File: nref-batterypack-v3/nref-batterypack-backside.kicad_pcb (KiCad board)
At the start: 2 copper layers, 75 x 17 mm, 8 parts, among them J1 C1+, J2 C2-, J3 C3+, J4 C4-, J5 FRONT_CONN

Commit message: battpack v3 snapshot
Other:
- board text added: "TODO: 4 layers to ensure thickness!"
- board text added: "TODO: fix holes etc"
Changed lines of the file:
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@@
 		(layer "Edge.Cuts")
+	)
+	(gr_text "TODO: fix holes etc"
+		(at 117.2 79.5 0)
+		(layer "Dwgs.User")
+		(effects
+			(font
+				(size 1 1)
+				(thickness 0.15)
+			)
+			(justify left bottom)
+		)
+	)
+	(gr_text "TODO: 4 layers to ensure thickness!"
+		(at 117.4 77.2 0)
+		(layer "Dwgs.User")
+		(effects
+			(font
+				(size 1 1)
+				(thickness 0.15)
+			)
+			(justify left bottom)
+		)
 	)
 	(segment

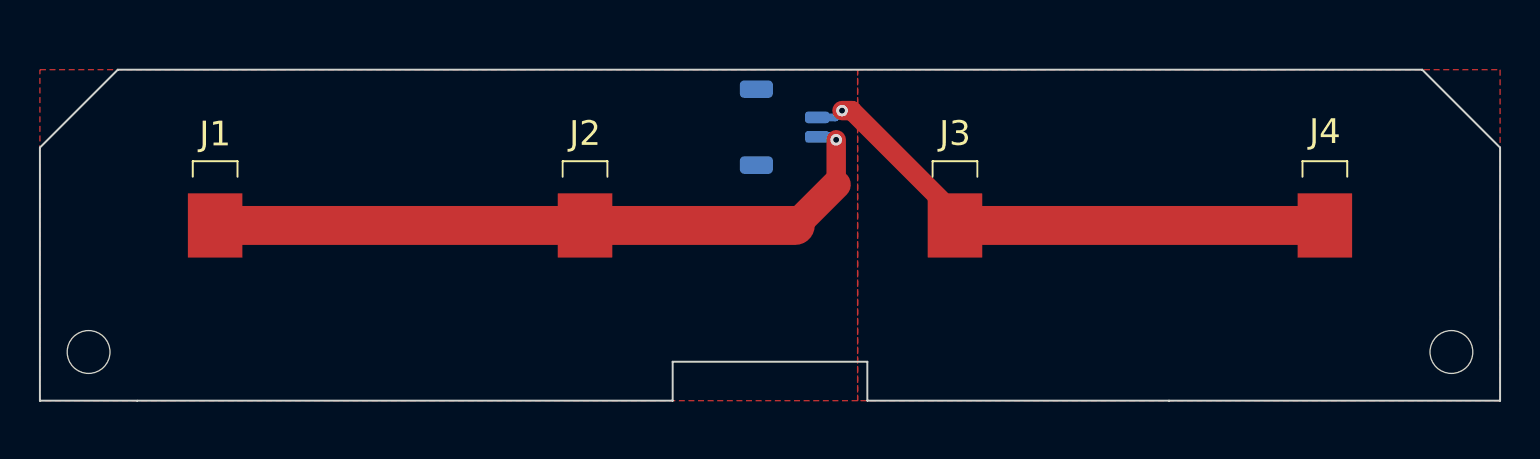
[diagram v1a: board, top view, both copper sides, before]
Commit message: batterypack v3 front+back pcbs polished for ordering
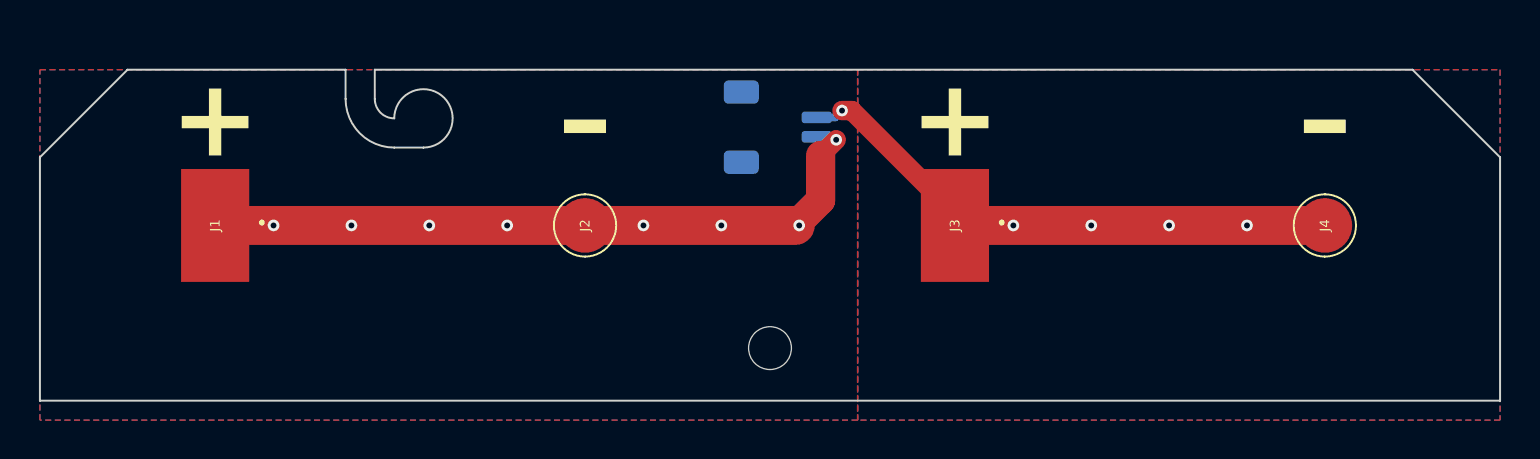
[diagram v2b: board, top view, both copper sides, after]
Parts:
- removed H2: MountingHole, MountingHole:MountingHole_2.2mm_M2
- J1, J3: footprint footprints:S713145R -> footprints:S174146R
- J2, J4: footprint footprints:S713145R -> footprints:S70332002045R
- J5: footprint Connector_JST:JST_SHL_SM02B-SHLS-TF_1x02-1MP_P1.00mm_Horizontal -> Connector_JST:JST_SH_SM02B-SRSS-TB_1x02-1MP_P1.00mm_Horizontal
- moved H1 35.0 mm to (127.5, 97.3)
- moved H3 1.10 mm to (127.5, 92.2)
- moved J5 0.35 mm to (127.9, 86.0)
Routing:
- net /C3+: vias 1 -> 5
- net /C1+: vias 1 -> 8
- added copper zone on B.Cu, net /C1+
- added copper zone on In1.Cu, net /C1+
- added copper zone on In2.Cu, net /C1+
- added copper zone on B.Cu, net /C3+
- added copper zone on In1.Cu, net /C3+
- added copper zone on In2.Cu, net /C3+
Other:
- outline, holes or cut-outs redrawn
- copper layers 2 -> 4
- board text added: "+"
- board text added: "–"
- board text removed: "TODO: 4 layers to ensure thickness!"
- board text removed: "TODO: fix holes etc"
